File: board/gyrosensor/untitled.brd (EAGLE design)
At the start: 38 x 24 mm, 17 parts

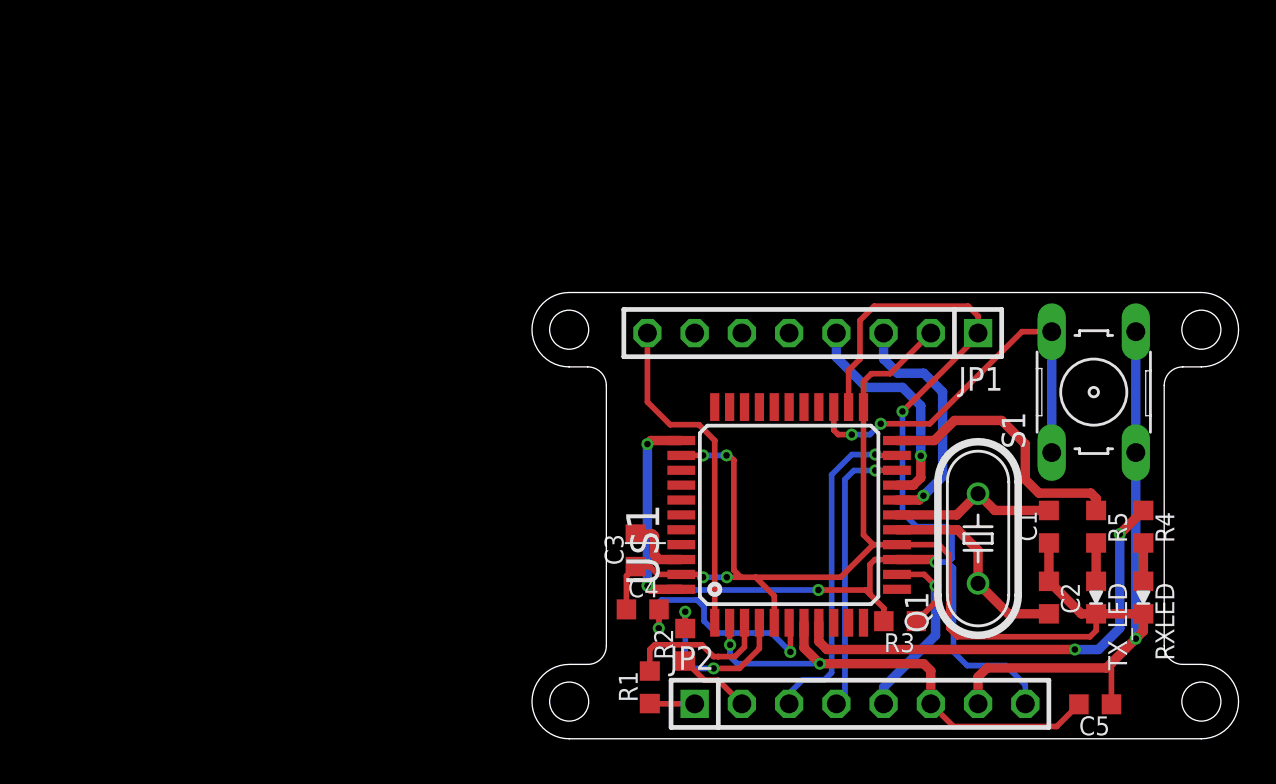
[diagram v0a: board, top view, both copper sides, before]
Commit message: Revert "Merge remote-tracking branch 'origin/Develop' into feature_#37"
This reverts commit cb103155361e8766478c6830db153463370c0739, reversing
changes made to 84e093fe944e1f8653a6822ff34e6f8740617cb5.
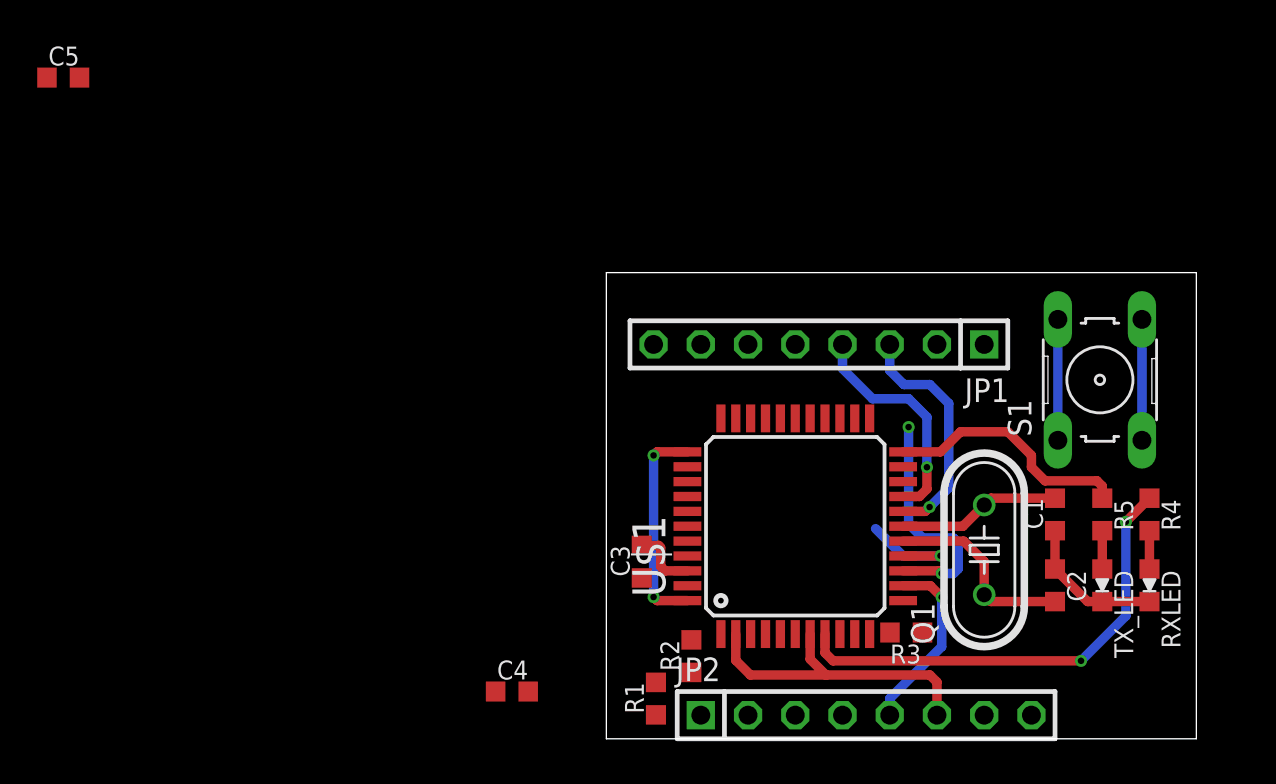
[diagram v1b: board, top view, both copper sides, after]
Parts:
- moved C5 64.9 mm to (-29.2, 35.6), turned to 0 degrees
- moved C4 8.31 mm to (-5.08, 2.54)
- moved RXLED 0.74 mm to (29.2, 8.26)
- moved TX_LED 0.74 mm to (26.7, 8.26)
- moved C2 0.74 mm to (24.1, 8.26)
- moved R4 0.74 mm to (29.2, 12.1)
- moved R5 0.74 mm to (26.7, 12.1)
- moved C1 0.74 mm to (24.1, 12.1)
- moved S1 0.74 mm to (26.5, 19.3)
- moved Q1 0.69 mm to (20.3, 10.2)
- moved R3 0.69 mm to (16.1, 5.71)
- moved JP2 0.69 mm to (14.0, 1.27)
- moved C3 0.69 mm to (1.91, 9.53)
- moved JP1 0.69 mm to (11.4, 21.2)
- moved R1 0.69 mm to (2.67, 2.16)
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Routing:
- net GND: track 98.5 -> 20.5 mm, vias 5 -> 1
- net VCC: track 70.8 -> 24.2 mm, vias 5 -> 4
- net INT: track 18.0 -> 0.00 mm
- net N$13: track 17.9 -> 0.00 mm, vias 1 -> 0
- net N$5: track 21.9 -> 6.50 mm, vias 2 -> 0
- net N$14: track 15.3 -> 0.00 mm, vias 1 -> 0
- net N$3: track 12.7 -> 0.00 mm, vias 2 -> 0
- net N$9: track 9.47 -> 0.00 mm, vias 2 -> 0
- net UVCC: track 26.2 -> 17.0 mm, vias 2 -> 0
- net N$8: track 8.14 -> 0.00 mm
- net D+: track 4.00 -> 0.00 mm
- net D-: track 2.42 -> 0.00 mm
- net RESET: track 12.2 -> 9.83 mm
- net N$7: track 14.7 -> 13.4 mm
- net N$6: track 24.7 -> 25.2 mm
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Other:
- board size 38 x 24 mm -> 31.7 x 25.1 mm

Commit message: complete gyro unit
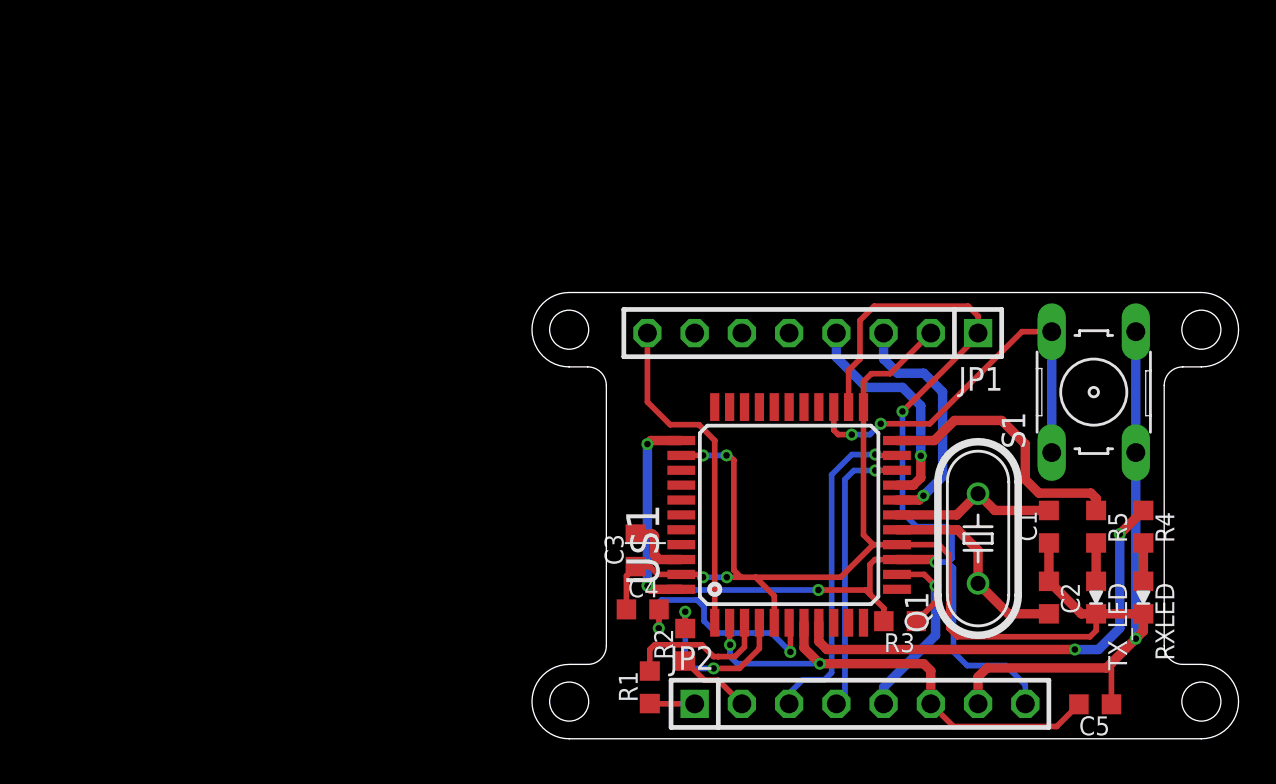
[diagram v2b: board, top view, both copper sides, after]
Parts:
- moved C5 64.9 mm to (26.3, 1.85), turned to 180 degrees
- moved C4 8.31 mm to (1.96, 6.96)
- moved RXLED 0.74 mm to (28.9, 7.59)
- moved TX_LED 0.74 mm to (26.3, 7.59)
- moved C2 0.74 mm to (23.8, 7.59)
- moved R4 0.74 mm to (28.9, 11.4)
- moved R5 0.74 mm to (26.3, 11.4)
- moved C1 0.74 mm to (23.8, 11.4)
- moved S1 0.74 mm to (26.2, 18.6)
- moved Q1 0.69 mm to (20.0, 10.8)
- moved R3 0.69 mm to (15.8, 6.32)
- moved JP2 0.69 mm to (13.6, 1.88)
- moved C3 0.69 mm to (1.57, 10.1)
- moved JP1 0.69 mm to (11.1, 21.8)
- moved R1 0.69 mm to (2.34, 2.77)
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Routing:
- net GND: track 20.5 -> 98.5 mm, vias 1 -> 5
- net VCC: track 24.2 -> 70.8 mm, vias 4 -> 5
- net INT: track 0.00 -> 18.0 mm
- net N$13: track 0.00 -> 17.9 mm, vias 0 -> 1
- net N$5: track 6.50 -> 21.9 mm, vias 0 -> 2
- net N$14: track 0.00 -> 15.3 mm, vias 0 -> 1
- net N$3: track 0.00 -> 12.7 mm, vias 0 -> 2
- net N$9: track 0.00 -> 9.47 mm, vias 0 -> 2
- net UVCC: track 17.0 -> 26.2 mm, vias 0 -> 2
- net N$8: track 0.00 -> 8.14 mm
- net D+: track 0.00 -> 4.00 mm
- net D-: track 0.00 -> 2.42 mm
- net RESET: track 9.83 -> 12.2 mm
- net N$7: track 13.4 -> 14.7 mm
- net N$6: track 25.2 -> 24.7 mm
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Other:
- board size 31.7 x 25.1 mm -> 38 x 24 mm
